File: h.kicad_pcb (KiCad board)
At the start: 2 copper layers, 4 parts, among them SW1 SW_Push, SW2 SW_Push, SW3 SW_Push, U1 MOUDLE-SEEEDUINO-XIAO

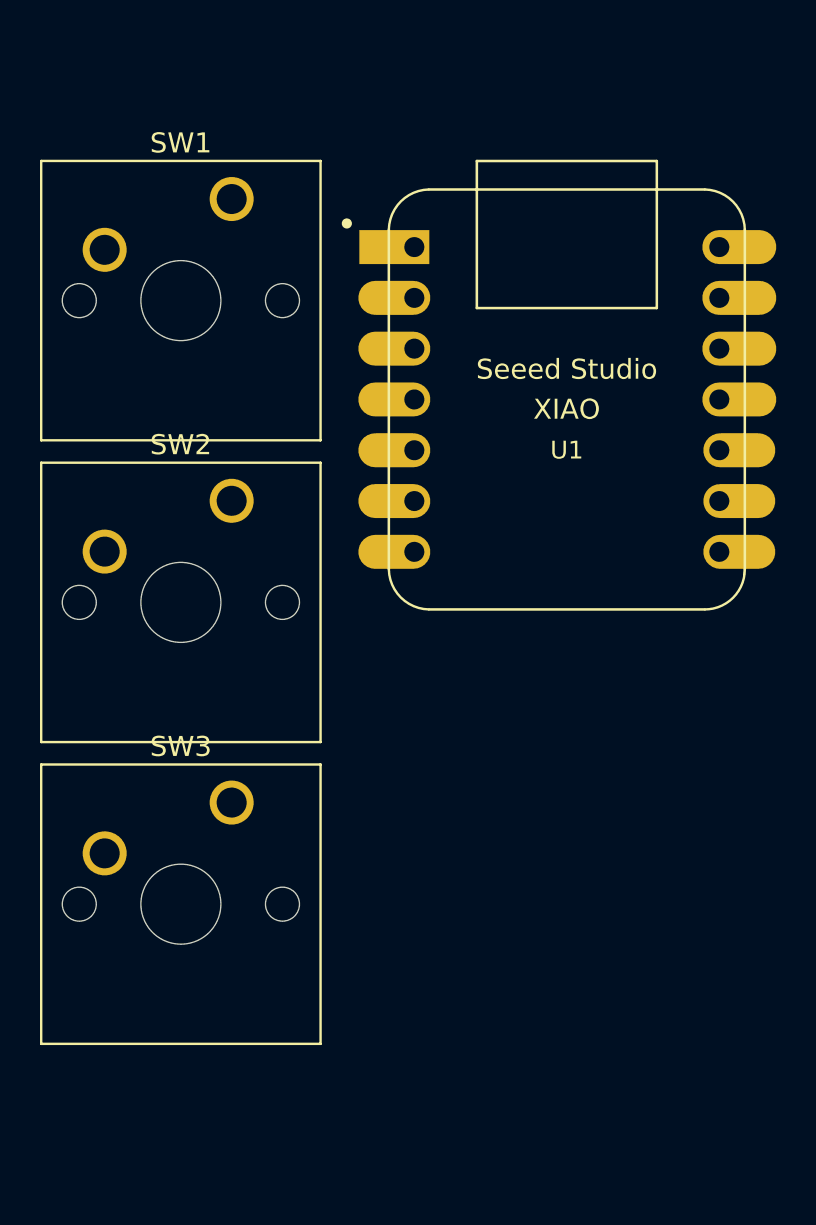
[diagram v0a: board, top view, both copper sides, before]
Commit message: and once more
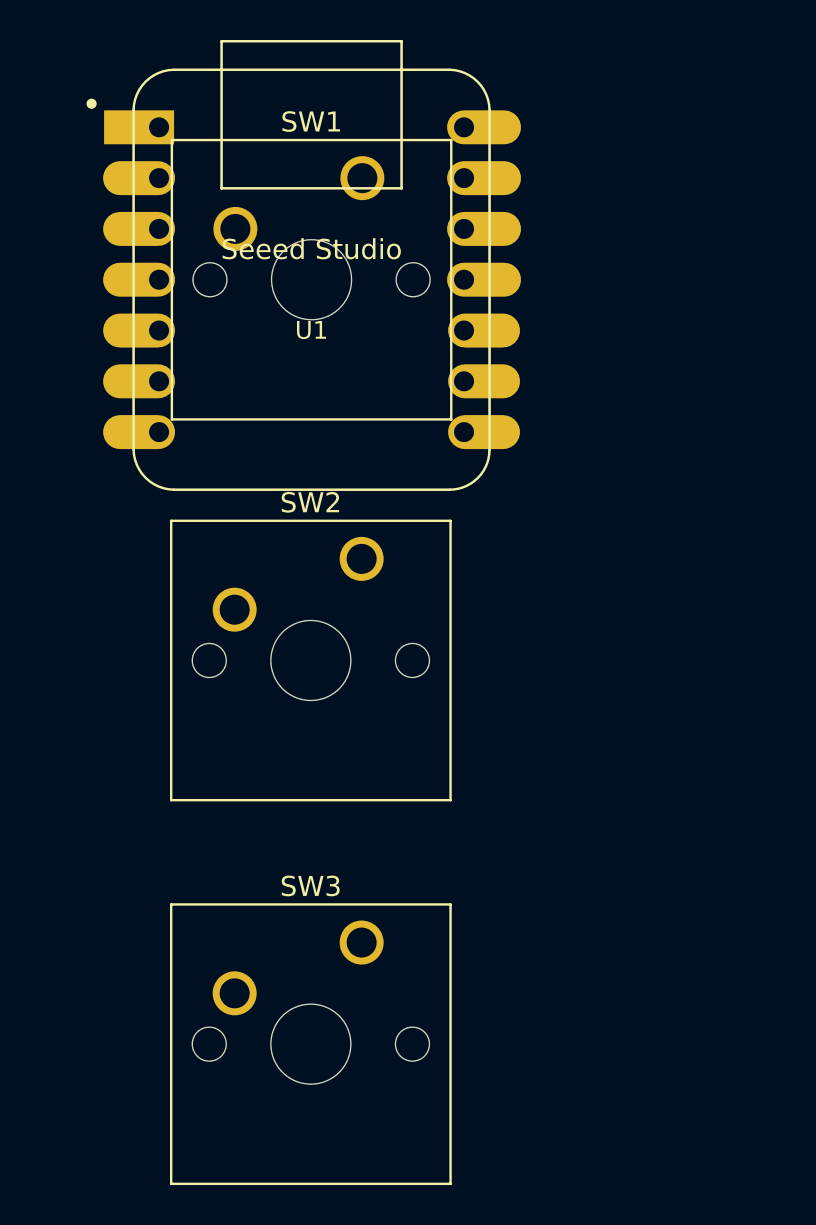
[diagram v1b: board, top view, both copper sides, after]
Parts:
- moved U1 14.1 mm to (144.1, 88.0)
- moved SW3 9.55 mm to (146.6, 121.1)
- moved SW2 7.12 mm to (146.6, 102.0)
- moved SW1 6.62 mm to (146.6, 82.9)
